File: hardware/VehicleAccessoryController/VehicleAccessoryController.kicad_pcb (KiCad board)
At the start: 2 copper layers, 61.4 x 75.2 mm, 79 parts, among them J501 Input, J502 Front Conn, J503 Rear Conn, J504 Left Conn, J505 Right Conn, J506 USB_B_Mini, P601 TC2030-MCP, Q201 BSS138, Q202 BSS138, Q203 BSS138, Q204 BSS138, SW301 ON/OFF, U101 RECOM_REMX0-W, U102 ATMEGA328P-M(32QFN_MLF), U103 TPS3710, U104 SI8710CC-B-IS, U105 CP2102N-A02-GQFN24, U106 Si8631EC-B-IS1, U107 NCV551SN50T1G, Y901 16MHz

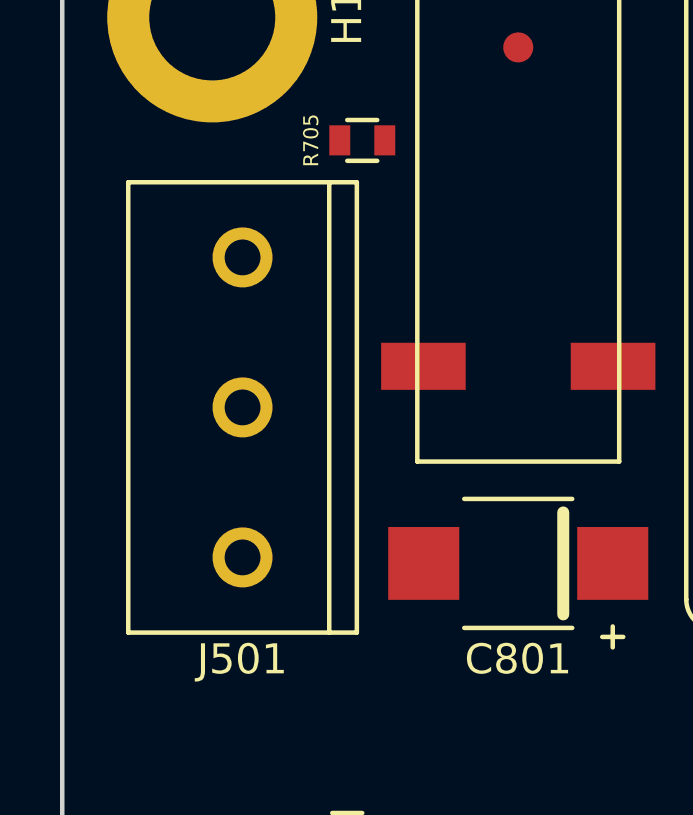
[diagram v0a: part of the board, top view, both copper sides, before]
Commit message: CAD models update
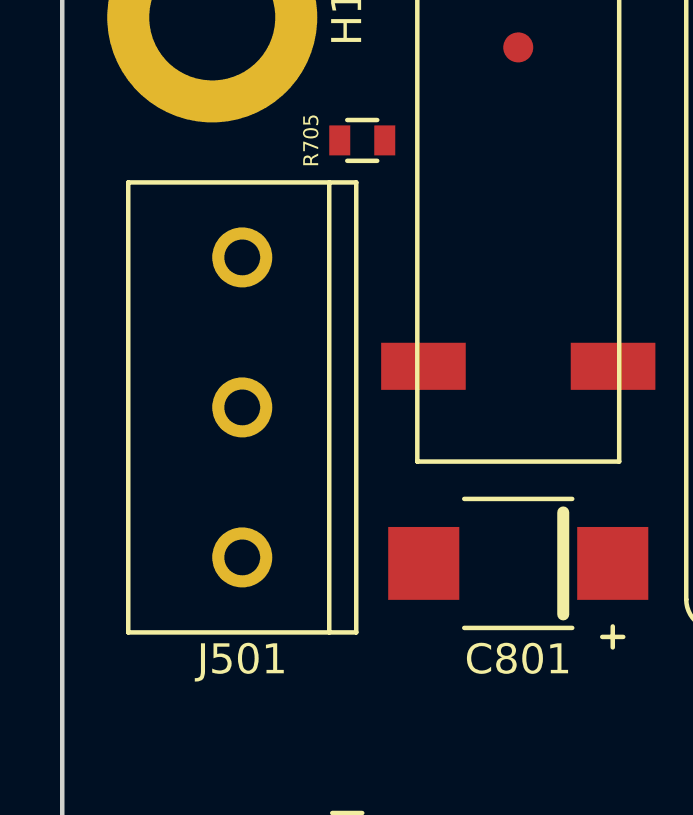
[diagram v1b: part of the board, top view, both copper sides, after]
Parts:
- U103: footprint VehicleAccessoryController:TI DSE (S-PWSON-N6) -> VehicleAccessoryController:TI_DSE_(S-PWSON-N6)
